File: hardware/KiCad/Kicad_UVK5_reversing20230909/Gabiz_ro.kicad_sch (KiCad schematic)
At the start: 66 parts, among them J37 Conn_Coaxial, Q08 24 NPN, Q23 24 NPN, Q9 R24 NPN, U3 C4_TLV70013_SOT23-5, U5 C4_TLV70013_SOT23-5, U6 C4_TLV70013_SOT23-5

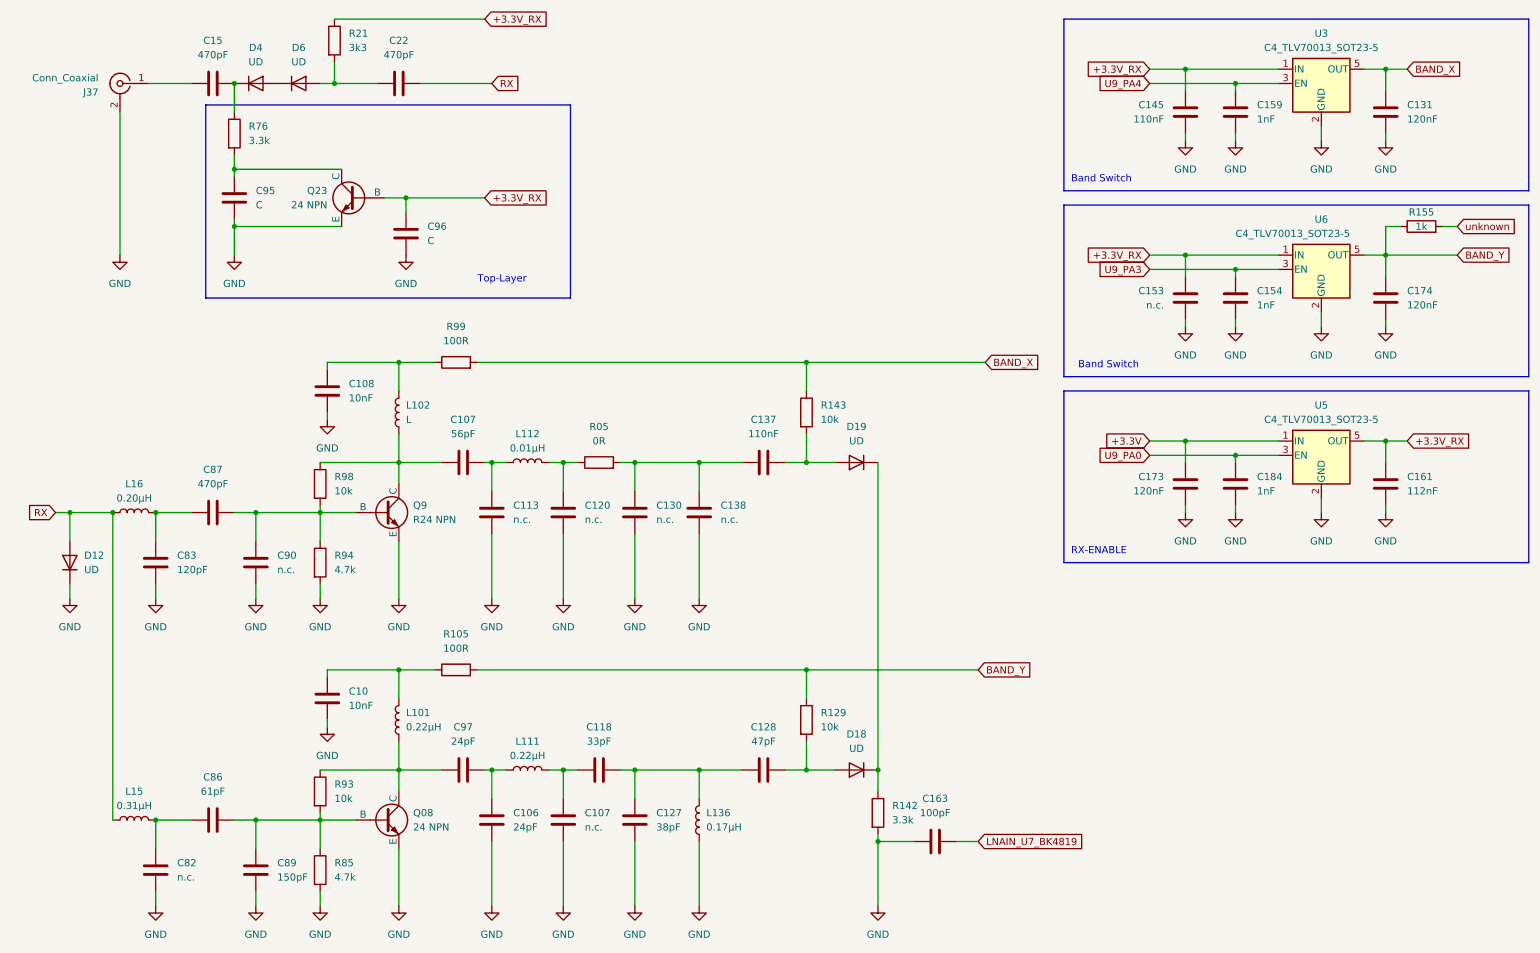
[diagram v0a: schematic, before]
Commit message: Add files via upload
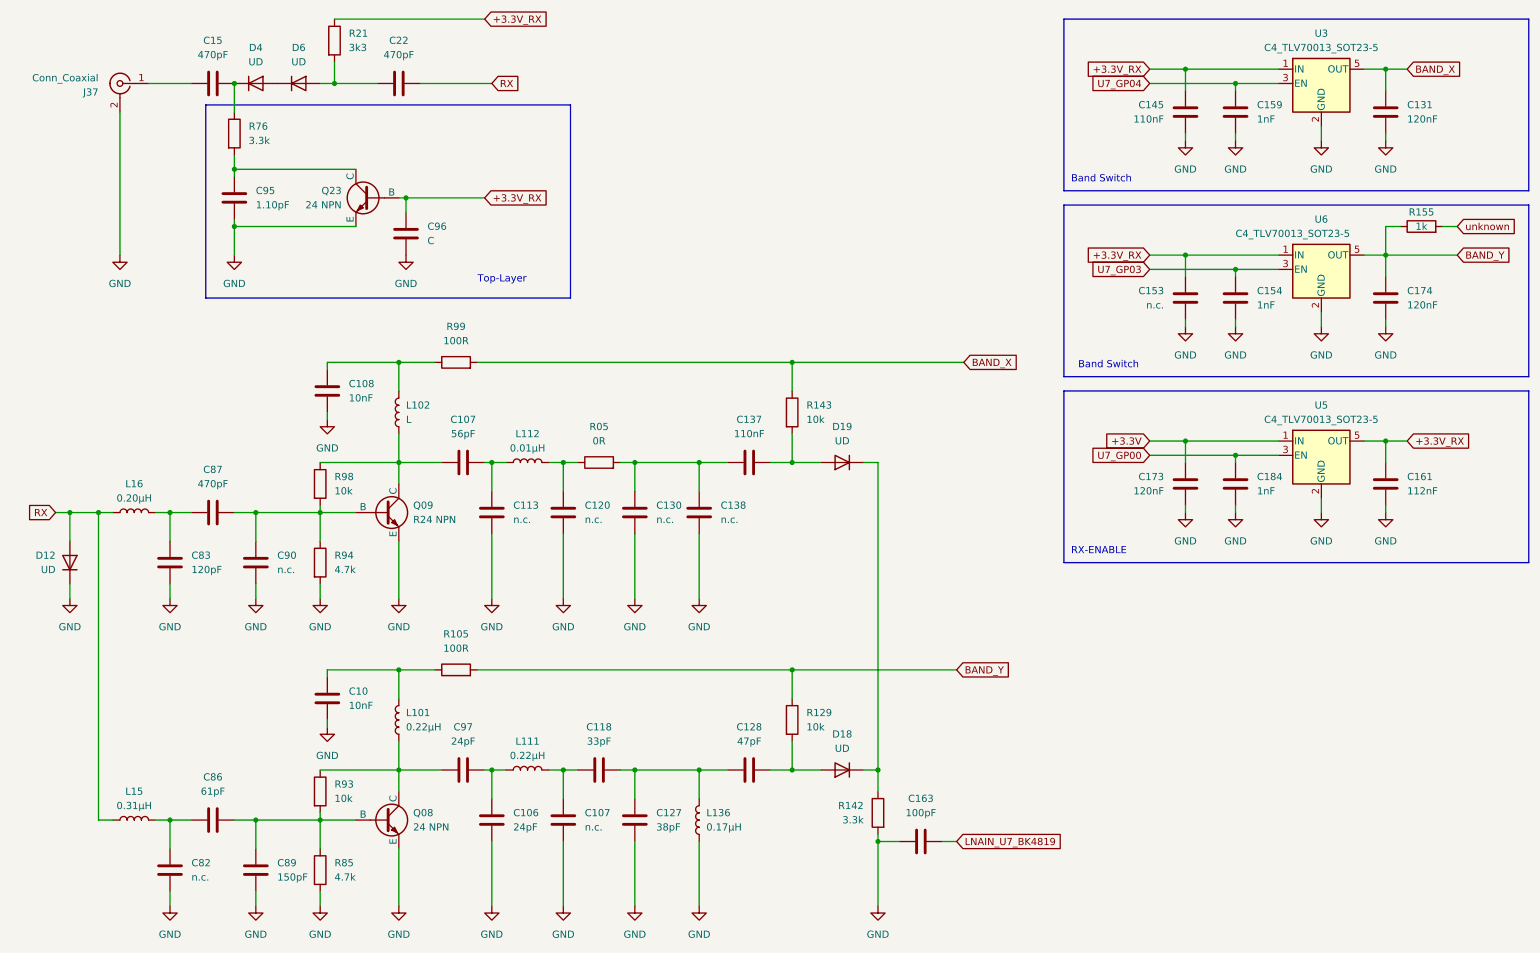
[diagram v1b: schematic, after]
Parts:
- C95: value C -> 1.10pF
- renumbered Q9 to Q09
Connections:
- net U9_PA0 renamed U7_GP00
- net U9_PA3 renamed U7_GP03
- net U9_PA4 renamed U7_GP04
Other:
- moved on the sheet: C128, C137, C163, C82, C83, D12, D18, D19, Q23, R129, R143
